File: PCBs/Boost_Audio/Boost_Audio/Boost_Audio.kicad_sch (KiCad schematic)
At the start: 42 parts, among them J1 XT60-M, J3 RL_Audio_From_Main, J4 To_Speaker_L, J5 To_Speaker_R, M3 CSD17581Q3, M4 CSD17581Q3A, U1 LM4752TS, U2 LM5122MH/NOPB

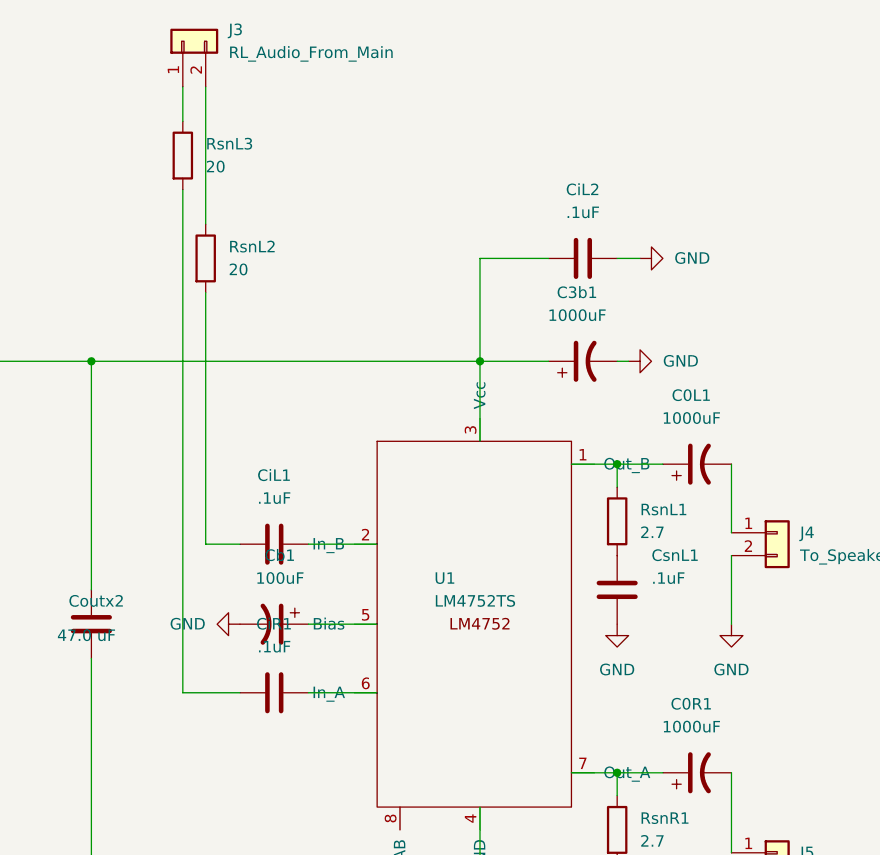
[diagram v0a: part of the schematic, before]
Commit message: latest PCBs
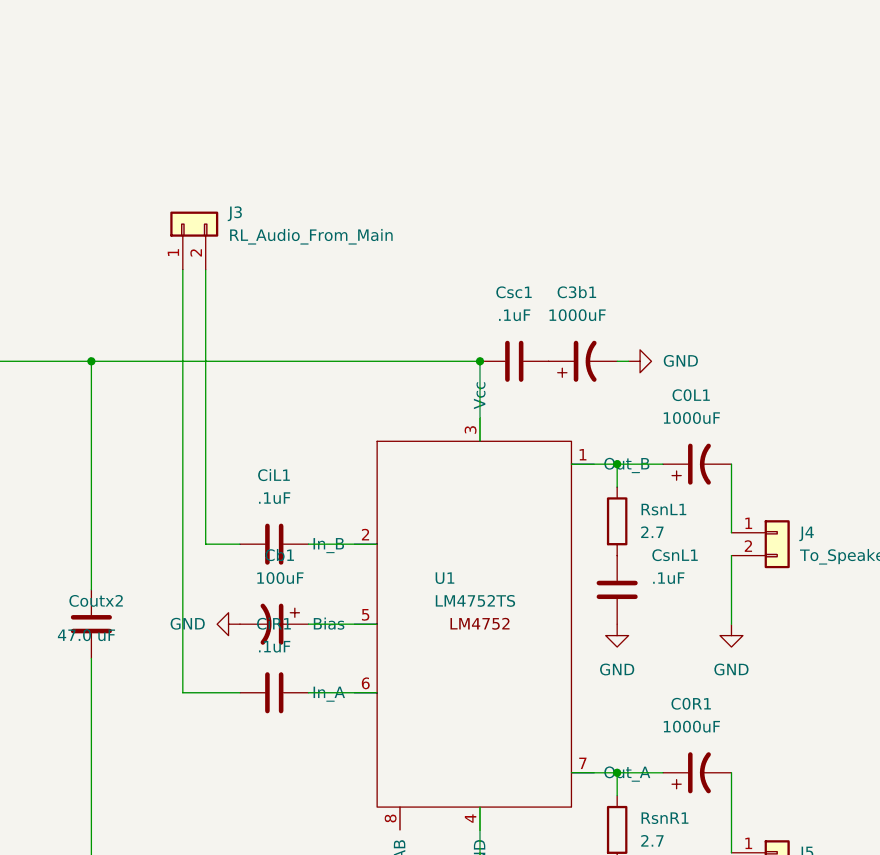
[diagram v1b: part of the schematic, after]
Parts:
- removed CiL2: .1uF, Capacitor_SMD:C_0805_2012Metric, symbol Device:C
- removed RsnL2, RsnL3: 20, Resistor_SMD:R_0805_2012Metric, symbol Device:R
- added Csc1: .1uF, Capacitor_SMD:C_0805_2012Metric, symbol Device:C
- Cbst2: footprint Artisyn_Components:CSD17309Q3 -> Capacitor_SMD:C_0805_2012Metric
- J3, J4, J5: footprint Connector_JST:JST_EH_B2B-EH-A_1x02_P2.50mm_Vertical -> Connector_PinHeader_2.54mm:PinHeader_1x02_P2.54mm_Vertical
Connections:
- net at Cout2.1, Coutx2.1, M4.5 (DRAIN)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: now also Csc1.1; no longer C3b1.1
- net at J3.1 (Pin_1): now also CiR1.1
- net at CiL1.1: now also J3.2 (Pin_2)
- new net: C3b1.1, Csc1.2
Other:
- moved on the sheet: J3
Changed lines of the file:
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@@
   (junction (at 34.29 67.31) (diameter 0) (color 0 0 0 0)
   )
+  (junction (at 246.38 67.31) (diameter 0) (color 0 0 0 0)
+  )
   (junction (at 175.26 72.39) (diameter 0) (color 0 0 0 0)
   )
@@
   (junction (at 175.26 69.85) (diameter 0) (color 0 0 0 0)
   )
-  (junction (at 246.38 67.31) (diameter 0) (color 0 0 0 0)
-  )
   (junction (at 54.61 132.08) (diameter 0) (color 0 0 0 0)
   )
@@
     (stroke (width 0) (type default))
   )
-  (wire (pts (xy 261.62 55.88) (xy 264.16 55.88))
-    (stroke (width 0) (type default))
-  )
   (wire (pts (xy 110.49 115.57) (xy 120.65 115.57))
     (stroke (width 0) (type default))
@@
     (stroke (width 0) (type default))
   )
-  (wire (pts (xy 246.38 55.88) (xy 246.38 67.31))
-    (stroke (width 0) (type default))
-  )
   (wire (pts (xy 203.2 67.31) (xy 203.2 92.71))
     (stroke (width 0) (type default))
@@
     (stroke (width 0) (type default))
   )
-  (wire (pts (xy 215.9 36.83) (xy 215.9 52.07))
-    (stroke (width 0) (type default))
-  )
   (wire (pts (xy 34.29 132.08) (xy 40.64 132.08))
     (stroke (width 0) (type default))
@@
     (stroke (width 0) (type default))
   )
-  (wire (pts (xy 213.36 36.83) (xy 213.36 40.64))
-    (stroke (width 0) (type default))
-  )
   (wire (pts (xy 110.49 95.25) (xy 128.27 95.25))
     (stroke (width 0) (type default))
@@
     (stroke (width 0) (type default))
   )
-  (wire (pts (xy 246.38 55.88) (xy 254 55.88))
-    (stroke (width 0) (type default))
-  )
   (wire (pts (xy 74.93 92.71) (xy 73.66 92.71))
     (stroke (width 0) (type default))
@@
     (stroke (width 0) (type default))
   )
-  (wire (pts (xy 215.9 59.69) (xy 215.9 87.63))
-    (stroke (width 0) (type default))
-  )
   (wire (pts (xy 274.32 78.74) (xy 274.32 86.36))
     (stroke (width 0) (type default))
@@
     (stroke (width 0) (type default))
   )
-  (wire (pts (xy 246.38 67.31) (xy 254 67.31))
-    (stroke (width 0) (type default))
-  )
   (wire (pts (xy 58.42 100.33) (xy 58.42 67.31))
     (stroke (width 0) (type default))
@@
     (stroke (width 0) (type default))
   )
+  (wire (pts (xy 215.9 57.15) (xy 215.9 87.63))
+    (stroke (width 0) (type default))
+  )
   (wire (pts (xy 124.46 76.2) (xy 125.73 76.2))
     (stroke (width 0) (type default))
@@
     (stroke (width 0) (type default))
   )
+  (wire (pts (xy 213.36 57.15) (xy 213.36 104.14))
+    (stroke (width 0) (type default))
+  )
   (wire (pts (xy 74.93 80.01) (xy 74.93 87.63))
     (stroke (width 0) (type default))
@@
   )
   (wire (pts (xy 130.81 91.44) (xy 139.7 91.44))
-    (stroke (width 0) (type default))
-  )
-  (wire (pts (xy 213.36 48.26) (xy 213.36 104.14))
     (stroke (width 0) (type default))
   )
@@
         (path "/fd5b3421-9c2a-40d1-9fed-b28030b8ba38"
           (reference "Css2") (unit 1)
-        )
-      )
-    )
-  )
-  (symbol (lib_id "power:GND") (at 264.16 55.88 90) (unit 1)
-    (in_bom yes) (on_board yes) (dnp no) (fields_autoplaced)
-    (property "Reference" "#PWR013" (at 270.51 55.88 0)
-      (effects (font (size 1.27 1.27)) hide)
-    )
-    (property "Value" "GND" (at 267.97 55.88 90)
-      (effects (font (size 1.27 1.27)) (justify right))
-    )
-    (property "Footprint" "" (at 264.16 55.88 0)
-      (effects (font (size 1.27 1.27)) hide)
-    )
-    (property "Datasheet" "" (at 264.16 55.88 0)
-      (effects (font (size 1.27 1.27)) hide)
-    )
-    (pin "1")
-    (instances
-      (project "Boost_Audio"
-        (path "/fd5b3421-9c2a-40d1-9fed-b28030b8ba38"
-          (reference "#PWR013") (unit 1)
         )
       )
@@
     )
   )
-  (symbol (lib_id "Device:C") (at 257.81 55.88 90) (unit 1)
-    (in_bom yes) (on_board yes) (dnp no) (fields_autoplaced)
-    (property "Reference" "CiL2" (at 257.81 48.26 90)
-      (effects (font (size 1.27 1.27)))
-    )
-    (property "Value" ".1uF" (at 257.81 50.8 90)
-      (effects (font (size 1.27 1.27)))
-    )
-    (property "Footprint" "Capacitor_SMD:C_0805_2012Metric" (at 261.62 54.9148 0)
-      (effects (font (size 1.27 1.27)) hide)
-    )
-    (property "Datasheet" "~" (at 257.81 55.88 0)
-      (effects (font (size 1.27 1.27)) hide)
-    )
-    (pin "1")
-    (pin "2")
-    (instances
-      (project "Boost_Audio"
-        (path "/fd5b3421-9c2a-40d1-9fed-b28030b8ba38"
-          (reference "CiL2") (unit 1)
-        )
-      )
-    )
-  )
   (symbol (lib_id "Device:R") (at 40.64 121.92 0) (unit 1)
     (in_bom yes) (on_board yes) (dnp no) (fields_autoplaced)
@@
       (effects (font (size 1.27 1.27)) (justify left))
     )
-    (property "Footprint" "Connector_JST:JST_EH_B2B-EH-A_1x02_P2.50mm_Vertical" (at 279.4 121.92 0)
+    (property "Footprint" "Connector_PinHeader_2.54mm:PinHeader_1x02_P2.54mm_Vertical" (at 279.4 121.92 0)
       (effects (font (size 1.27 1.27)) hide)
     )
@@
     )
   )
-  (symbol (lib_id "Device:R") (at 213.36 44.45 0) (unit 1)
-    (in_bom yes) (on_board yes) (dnp no) (fields_autoplaced)
-    (property "Reference" "RsnL3" (at 215.9 43.18 0)
-      (effects (font (size 1.27 1.27)) (justify left))
-    )
-    (property "Value" "20" (at 215.9 45.72 0)
-      (effects (font (size 1.27 1.27)) (justify left))
-    )
-    (property "Footprint" "Resistor_SMD:R_0805_2012Metric" (at 211.582 44.45 90)
-      (effects (font (size 1.27 1.27)) hide)
-    )
-    (property "Datasheet" "~" (at 213.36 44.45 0)
-      (effects (font (size 1.27 1.27)) hide)
-    )
-    (pin "1")
-    (pin "2")
-    (instances
-      (project "Boost_Audio"
-        (path "/fd5b3421-9c2a-40d1-9fed-b28030b8ba38"
-          (reference "RsnL3") (unit 1)
-        )
-      )
-    )
-  )
   (symbol (lib_id "power:GND") (at 274.32 96.52 0) (unit 1)
     (in_bom yes) (on_board yes) (dnp no) (fields_autoplaced)
@@
     )
   )
+  (symbol (lib_id "Device:C") (at 250.19 67.31 90) (unit 1)
+    (in_bom yes) (on_board yes) (dnp no) (fields_autoplaced)
+    (property "Reference" "Csc1" (at 250.19 59.69 90)
+      (effects (font (size 1.27 1.27)))
+    )
+    (property "Value" ".1uF" (at 250.19 62.23 90)
+      (effects (font (size 1.27 1.27)))
+    )
+    (property "Footprint" "Capacitor_SMD:C_0805_2012Metric" (at 254 66.3448 0)
+      (effects (font (size 1.27 1.27)) hide)
+    )
+    (property "Datasheet" "~" (at 250.19 67.31 0)
+      (effects (font (size 1.27 1.27)) hide)
+    )
+    (pin "2")
+    (pin "1")
+    (instances
+      (project "Boost_Audio"
+        (path "/fd5b3421-9c2a-40d1-9fed-b28030b8ba38"
+          (reference "Csc1") (unit 1)
+        )
+      )
+    )
+  )
   (symbol (lib_id "power:GND") (at 262.89 67.31 90) (unit 1)
     (in_bom yes) (on_board yes) (dnp no) (fields_autoplaced)
@@
       (effects (font (size 1.27 1.27)) (justify left))
     )
-    (property "Footprint" "Connector_JST:JST_EH_B2B-EH-A_1x02_P2.50mm_Vertical" (at 279.4 86.36 0)
+    (property "Footprint" "Connector_PinHeader_2.54mm:PinHeader_1x02_P2.54mm_Vertical" (at 279.4 86.36 0)
       (effects (font (size 1.27 1.27)) hide)
     )
@@
       (effects (font (size 1.27 1.27)))
     )
-    (property "Footprint" "Artisyn_Components:CSD17309Q3" (at 106.68 71.4248 0)
+    (property "Footprint" "Capacitor_SMD:C_0805_2012Metric" (at 106.68 71.4248 0)
       (effects (font (size 1.27 1.27)) hide)
     )
@@
     )
   )
-  (symbol (lib_id "Device:R") (at 215.9 55.88 0) (unit 1)
-    (in_bom yes) (on_board yes) (dnp no) (fields_autoplaced)
-    (property "Reference" "RsnL2" (at 218.44 54.61 0)
-      (effects (font (size 1.27 1.27)) (justify left))
-    )
-    (property "Value" "20" (at 218.44 57.15 0)
-      (effects (font (size 1.27 1.27)) (justify left))
-    )
-    (property "Footprint" "Resistor_SMD:R_0805_2012Metric" (at 214.122 55.88 90)
-      (effects (font (size 1.27 1.27)) hide)
-    )
-    (property "Datasheet" "~" (at 215.9 55.88 0)
-      (effects (font (size 1.27 1.27)) hide)
-    )
-    (pin "1")
-    (pin "2")
-    (instances
-      (project "Boost_Audio"
-        (path "/fd5b3421-9c2a-40d1-9fed-b28030b8ba38"
-          (reference "RsnL2") (unit 1)
-        )
-      )
-    )
-  )
-  (symbol (lib_id "Connector_Generic:Conn_01x02") (at 213.36 31.75 90) (unit 1)
-    (in_bom yes) (on_board yes) (dnp no) (fields_autoplaced)
-    (property "Reference" "J3" (at 218.44 30.48 90)
+  (symbol (lib_id "Connector_Generic:Conn_01x02") (at 213.36 52.07 90) (unit 1)
+    (in_bom yes) (on_board yes) (dnp no) (fields_autoplaced)
+    (property "Reference" "J3" (at 218.44 50.8 90)
       (effects (font (size 1.27 1.27)) (justify right))
     )
-    (property "Value" "RL_Audio_From_Main" (at 218.44 33.02 90)
+    (property "Value" "RL_Audio_From_Main" (at 218.44 53.34 90)
       (effects (font (size 1.27 1.27)) (justify right))
     )
-    (property "Footprint" "Connector_JST:JST_EH_B2B-EH-A_1x02_P2.50mm_Vertical" (at 213.36 31.75 0)
-      (effects (font (size 1.27 1.27)) hide)
-    )
-    (property "Datasheet" "~" (at 213.36 31.75 0)
-      (effects (font (size 1.27 1.27)) hide)
-    )
+    (property "Footprint" "Connector_PinHeader_2.54mm:PinHeader_1x02_P2.54mm_Vertical" (at 213.36 52.07 0)
+      (effects (font (size 1.27 1.27)) hide)
+    )
+    (property "Datasheet" "~" (at 213.36 52.07 0)
+      (effects (font (size 1.27 1.27)) hide)
+    )
